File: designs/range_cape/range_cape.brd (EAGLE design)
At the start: 37 parts, among them J1 22-05-7048-04, J10 22-05-7048-04, J11 22-05-7048-04, J12 22-05-7048-04, J2 22-05-7048-04, J3 22-05-7048-04, J4 22-05-7048-04, J5 22-05-7048-04, J6 22-05-7048-04, J7 22-05-7048-04, J8 22-05-7048-04, J9 22-05-7048-04, U5 LMS8117AMP-3.3, U6 MSP430FR5739IDA

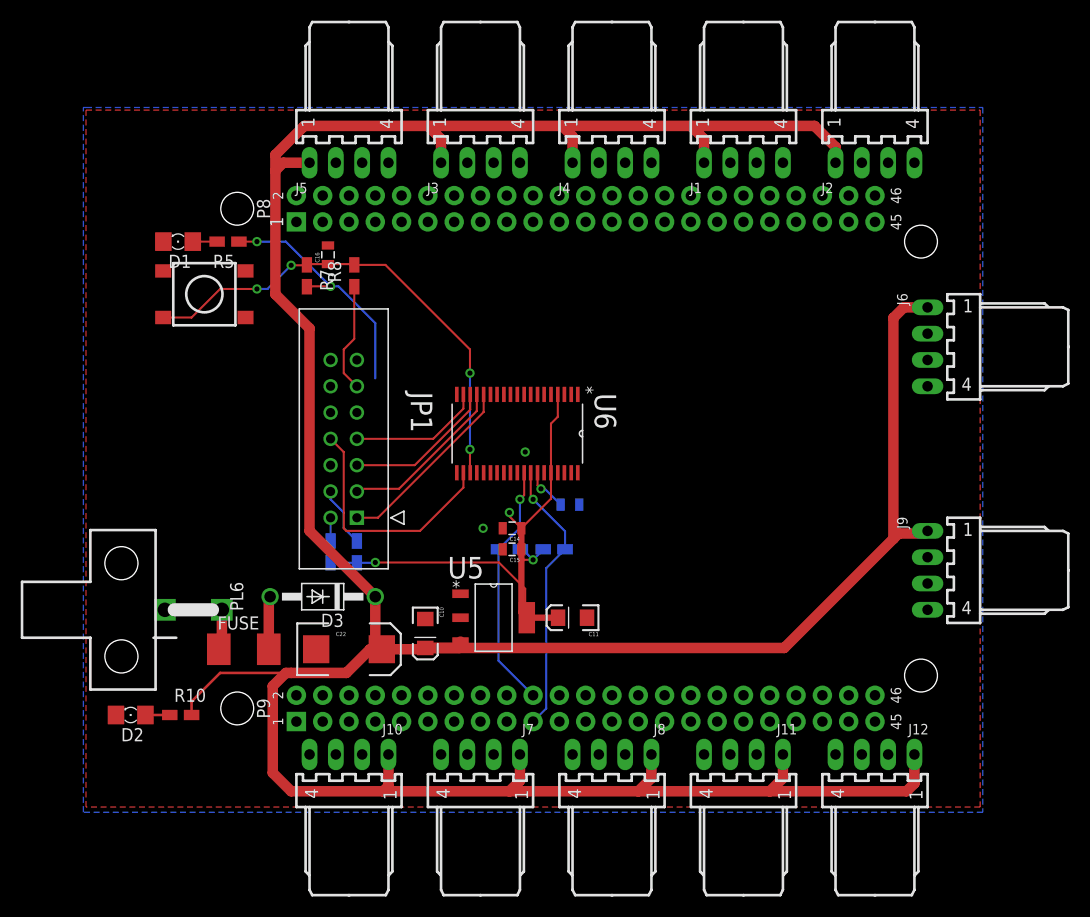
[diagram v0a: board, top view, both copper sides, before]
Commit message: done with range cape
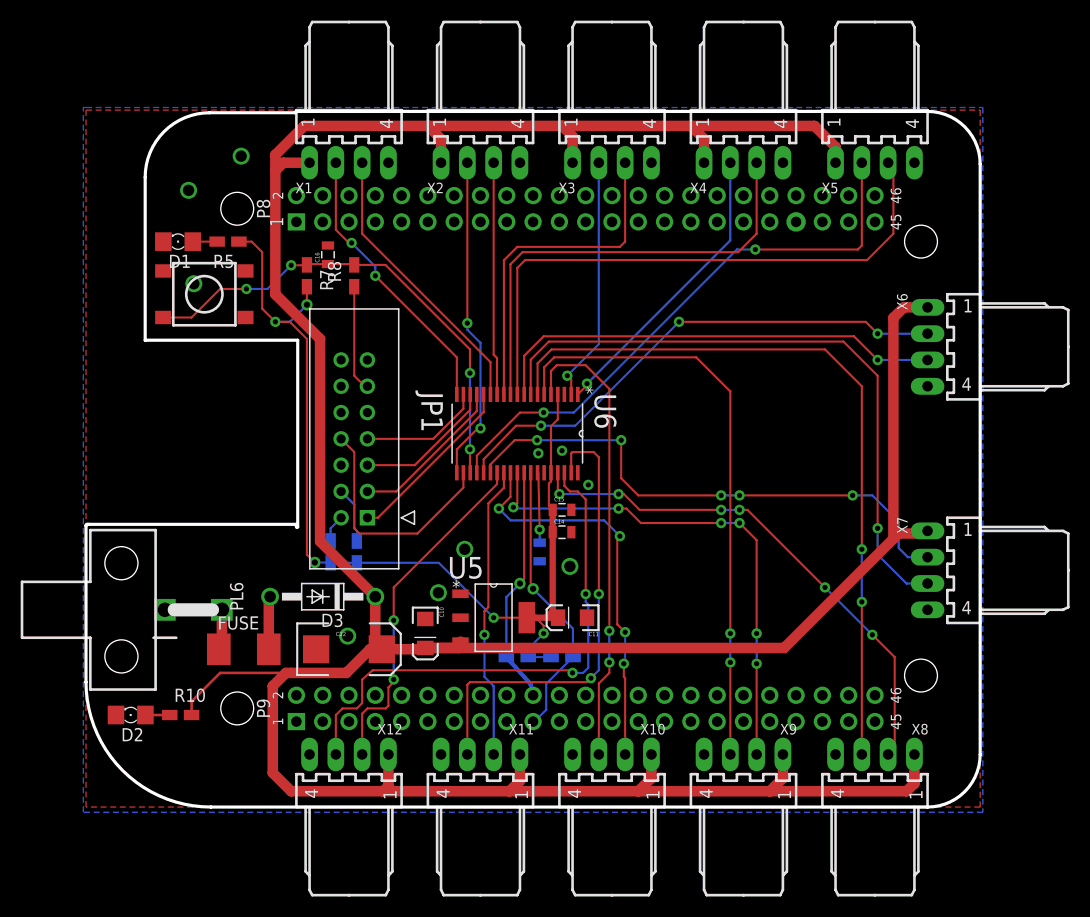
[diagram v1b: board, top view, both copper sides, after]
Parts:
- moved R2 10.4 mm to (41.7, 8.13)
- moved R1 10.4 mm to (46.0, 8.13)
- moved C15 6.15 mm to (46.0, 22.4), turned to 0 degrees
- moved C12 5.43 mm to (43.8, 18.3), turned to 90 degrees
- moved C14 4.84 mm to (46.0, 20.2), turned to 0 degrees
- moved JP1 1.02 mm to (24.6, 21.6)
- renumbered J1 to X4, J10 to X12, J11 to X9, J12 to X8, J2 to X5, J3 to X2, J4 to X3, J5 to X1, J6 to X6, J7 to X11, J8 to X10, J9 to X7
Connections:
- removed net N$10: X11.2
- removed net N$11: X10.2
- removed net N$12: X10.3
- removed net N$18: X7.2
- removed net N$19: X7.3
- removed net N$22: X12.2
- removed net N$23: X12.3
- removed net N$26: X9.2
- removed net N$27: X9.3
- removed net N$30: X8.2
- removed net N$31: X8.3
- removed net N$34: X6.3
- removed net N$35: X6.2
- removed net N$41: X1.3
- removed net N$42: X1.2
- removed net N$43: X3.3
- removed net N$44: X3.2
- removed net N$46: X2.3
- removed net N$47: X2.2
- removed net N$50: X5.3
- removed net N$51: X5.2
- removed net N$54: X4.3
- removed net N$55: X4.2
- removed net N$7: X11.3
- new net MSP_ADC0: U6.5, X10.3
- new net MSP_ADC1: U6.6, X9.3
- new net MSP_ADC12: U6.8, X7.3
- new net MSP_ADC13: U6.9, X6.3
- new net MSP_ADC14: U6.10, X5.3
- new net MSP_ADC15: U6.11, X4.3
- new net MSP_ADC2: U6.7, X8.3
- new net MSP_ADC5: U6.14, X1.3
- new net MSP_ADC6: U6.36, X12.3
- new net MSP_ADC7: U6.37, X11.3
- new net X-1: U6.19, X1.2
- new net X-10: U6.28, X10.2
- new net X-11: U6.27, X11.2
- new net X-12: U6.26, X12.2
- new net X-2: U6.20, X2.2
- new net X-3: U6.2, X3.2
- new net X-4: U6.1, X4.2
- new net X-5: U6.23, X5.2
- new net X-6: U6.24, X6.2
- new net X-7: U6.25, X7.2
- new net X-8: U6.35, X8.2
- new net X-9: U6.29, X9.2
- net MSP_ADC3: now also X3.3
- net MSP_ADC4: now also X2.3
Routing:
- net MSP_ADC2: track 0.00 -> 71.9 mm, vias 0 -> 2
- net MSP_ADC12: track 0.00 -> 62.2 mm, vias 0 -> 1
- net MSP_ADC1: track 0.00 -> 57.4 mm, vias 0 -> 2
- net MSP_ADC14: track 0.00 -> 57.0 mm
- net X-5: track 0.00 -> 55.2 mm, vias 0 -> 2
- net X-7: track 0.00 -> 52.3 mm, vias 0 -> 5
- net MSP_ADC6: track 0.00 -> 51.8 mm, vias 0 -> 2
- net X-8: track 0.00 -> 50.9 mm, vias 0 -> 6
- net X-6: track 0.00 -> 50.2 mm, vias 0 -> 3
- net X-9: track 0.00 -> 49.0 mm, vias 0 -> 6
- net MSP_ADC7: track 0.00 -> 45.4 mm, vias 0 -> 2
- net MSP_ADC0: track 0.00 -> 44.8 mm, vias 0 -> 2
- net MSP_ADC15: track 0.00 -> 44.4 mm
- net MSP_ADC13: track 0.00 -> 44.4 mm, vias 0 -> 1
- net X-10: track 0.00 -> 38.3 mm, vias 0 -> 4
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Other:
- board outline added: 86.4 x 67.2 mm
